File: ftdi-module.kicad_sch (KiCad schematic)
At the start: 58 parts, among them U1 AP62301_TSOT, U2 FT4232H_VQFN, U3 AP62301_TSOT, Y1 Resonator_12MHz_ABM8G

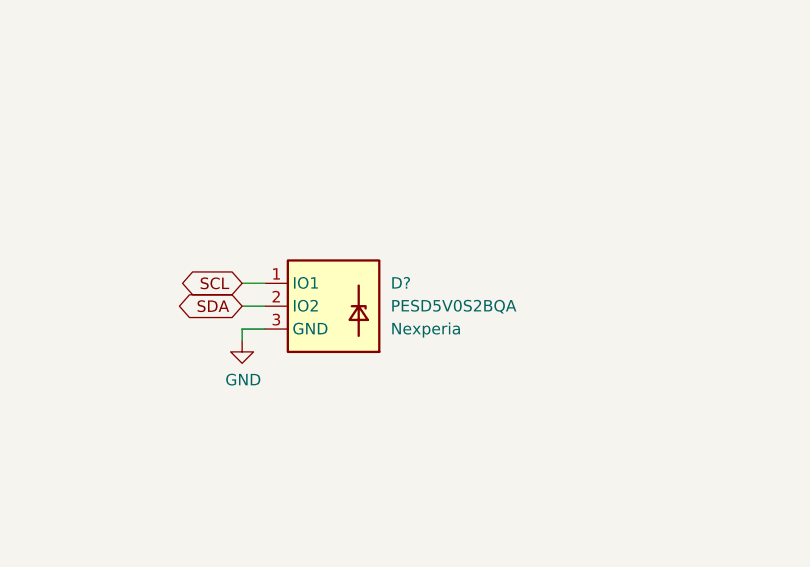
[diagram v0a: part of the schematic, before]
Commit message: Next batch of standardization
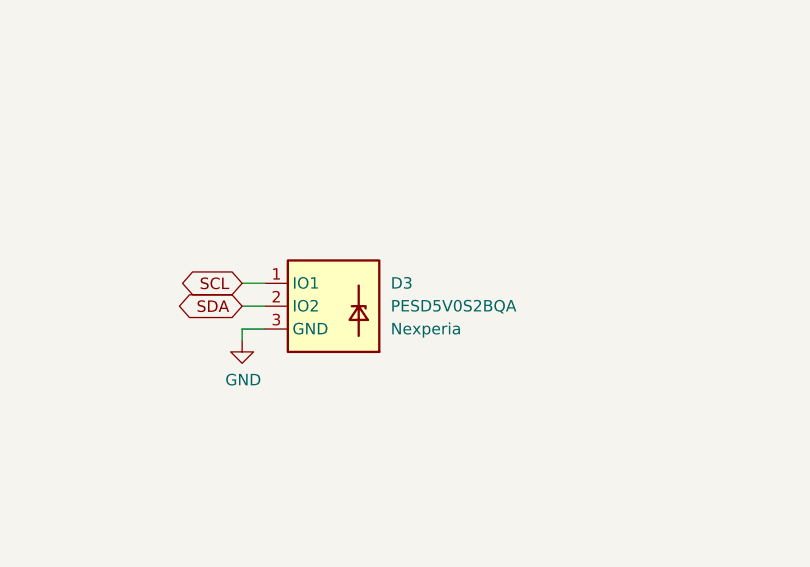
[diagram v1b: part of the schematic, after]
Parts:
- gave numbers to parts that had none: 1
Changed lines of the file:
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@@
   (symbol (lib_name "PESD5V0S2BQA_1") (lib_id "antmicroTVSDiodes:PESD5V0S2BQA") (at 255.27 53.34 0) (unit 1)
     (in_bom yes) (on_board yes) (fields_autoplaced)
-    (property "Reference" "D?" (id 0) (at 269.24 53.3399 0)
+    (property "Reference" "D3" (id 0) (at 269.24 53.3399 0)
       (effects (font (size 1.27 1.27) (thickness 0.15)) (justify left))
     )
